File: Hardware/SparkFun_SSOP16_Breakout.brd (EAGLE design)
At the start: 25.4 x 12.7 mm, 4 parts, among them U1 SSOP16

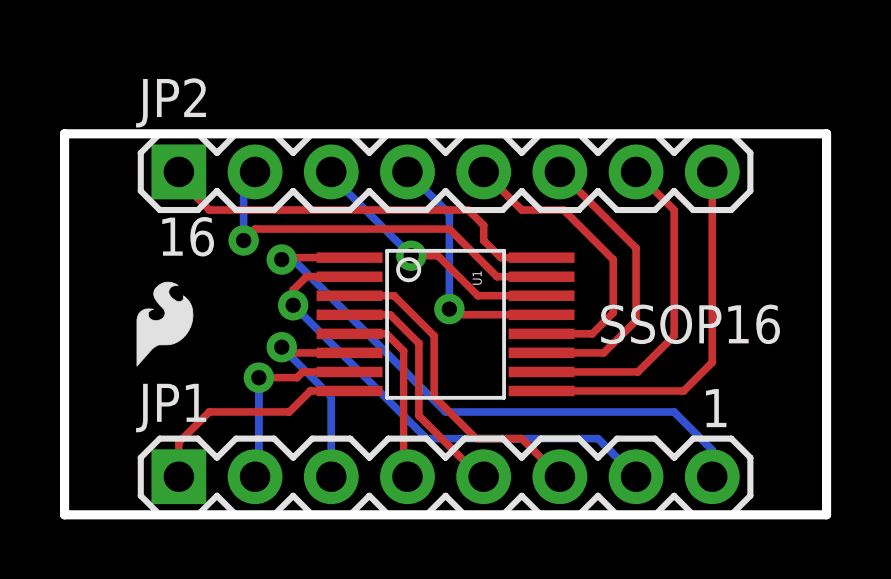
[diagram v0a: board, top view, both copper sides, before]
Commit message: Updated board files
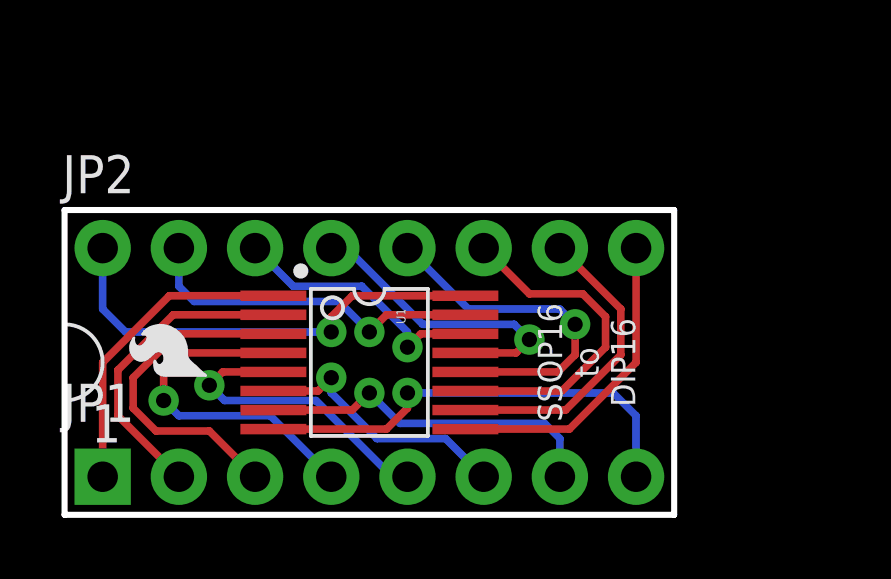
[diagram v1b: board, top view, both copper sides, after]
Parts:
- removed U$1: LOGO-SFESK, SparkFun:SFE-LOGO-FLAME
- added FRAME1: FRAME-LETTER, SparkFun-Aesthetics:CREATIVE_COMMONS
- added LOGO1: SFE_LOGO_FLAME.1_INCH, SparkFun-Aesthetics:SFE_LOGO_FLAME_.1
- added LOGO3: OSHW-LOGOS, SparkFun-Aesthetics:OSHW-LOGO-S
- JP1: device SparkFun:1X08 -> SparkFun-Connectors:1X08_PIN1_NO_SILK
- JP2: device SparkFun:1X08 -> SparkFun-Connectors:1X08_NO_SILK
- U1: device SparkFun:SSOP16 -> generic-ssop16:SSOP16
- moved JP2 3.59 mm to (1.27, 8.89)
- moved U1 2.84 mm to (10.2, 5.08)
- moved JP1 2.54 mm to (1.27, 1.27)
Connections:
- net N$1: now also U1.P$1; no longer U1.P$8
- net N$2: now also U1.P$2; no longer U1.P$7
- net N$3: now also U1.P$3; no longer U1.P$6
- net N$4: now also U1.P$4; no longer U1.P$5
- net N$5: now also U1.P$5; no longer U1.P$4
- net N$6: now also U1.P$6; no longer U1.P$3
- net N$7: now also U1.P$7; no longer U1.P$2
- net N$8: now also U1.P$8; no longer U1.P$1
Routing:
- net N$4: track 6.28 -> 11.6 mm, vias 0 -> 1
- net N$8: track 20.2 -> 15.2 mm
- net N$7: track 16.4 -> 11.7 mm
- net N$2: track 6.46 -> 10.3 mm, vias 1 -> 0
- net N$3: track 7.52 -> 11.3 mm, vias 1 -> 0
- net N$1: track 7.67 -> 10.4 mm
- net N$5: track 8.12 -> 10.2 mm, vias 0 -> 1
- net N$16: track 12.4 -> 10.4 mm
- net N$12: track 8.30 -> 10.2 mm
- net N$6: track 10.7 -> 8.86 mm, vias 0 -> 1
- net N$14: track 9.60 -> 11.3 mm
- net N$13: track 9.98 -> 11.6 mm, vias 0 -> 1
- net N$10: track 13.2 -> 11.7 mm
- net N$9: track 13.8 -> 15.2 mm, vias 0 -> 1
- net N$15: track 10.9 -> 10.3 mm
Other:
- board size 25.4 x 12.7 mm -> 20.3 x 10.2 mm
- board text added: "Byron Jacquot"
- board text added: "SSOP16 to DIP16"
- board text removed: "16"
- board text removed: "SSOP16"
